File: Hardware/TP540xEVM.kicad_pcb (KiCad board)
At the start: 2 copper layers, 27.9 x 20.3 mm, 11 parts, among them U1 TPS5403

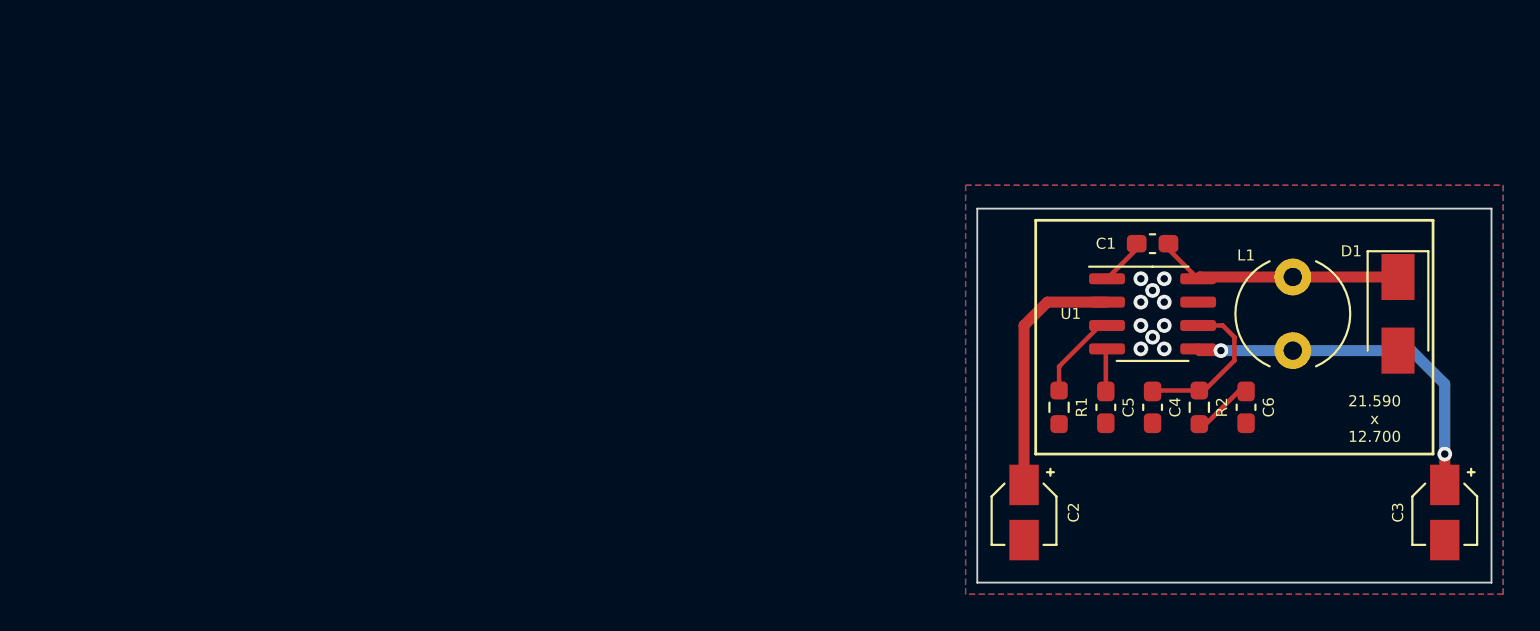
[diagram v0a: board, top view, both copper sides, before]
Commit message: ...
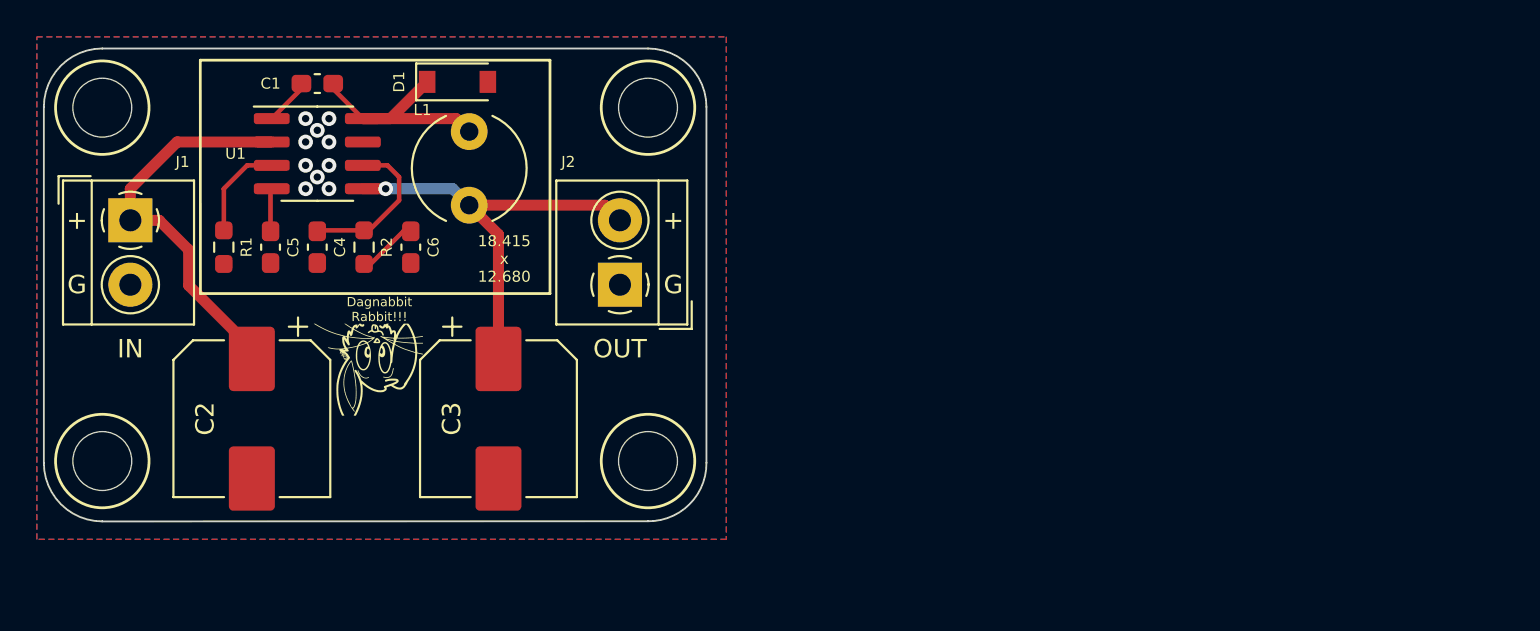
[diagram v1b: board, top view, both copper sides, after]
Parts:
- added J1: Input, TerminalBlock_4Ucon:TerminalBlock_4Ucon_1x02_P3.50mm_Horizontal, F.Cu at (86.7, 96.5)
- added J2: Output, TerminalBlock_4Ucon:TerminalBlock_4Ucon_1x02_P3.50mm_Horizontal, F.Cu at (113.3, 100.0)
- added REF**: Mount, Tinker:Mount, F.Cu at (114.8, 109.6)
- added REF**: Mount, Tinker:Mount, F.Cu at (85.2, 90.4)
- added REF**: Mount, Tinker:Mount, F.Cu at (85.2, 109.6)
- added REF**: DagNabbit, Tinker:DagNabbit, F.Cu at (99.9, 104.0)
- added REF**: Mount, Tinker:Mount, F.Cu at (114.8, 90.4)
- C2, C3: value 220uF -> 330uF; footprint Capacitor_SMD:CP_Elec_3x5.3 -> Capacitor_SMD:CP_Elec_8x10
- D1: value D_Schottky -> DSK24; footprint Diode_SMD:D_SMA -> Diode_SMD:D_SOD-123
- moved D1 52.6 mm to (104.5, 89.0), turned to 0 degrees
- moved C3 51.7 mm to (106.7, 107.3)
- moved C1 46.2 mm to (96.9, 89.1)
- moved C4 46.2 mm to (96.9, 98.0)
- moved R2 46.2 mm to (99.4, 98.0)
- moved U1 46.2 mm to (96.9, 92.9)
- moved C5 46.2 mm to (94.3, 98.0)
- moved C6 46.2 mm to (101.9, 98.0)
- moved R1 46.2 mm to (91.8, 98.0)
- moved L1 45.4 mm to (105.1, 91.7)
- moved C2 42.3 mm to (93.3, 107.3)
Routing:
- net Vin: track 13.7 -> 21.4 mm
- net Vout: track 19.7 -> 23.7 mm, vias 2 -> 1
- net Net-(R1-Pad1): track 4.83 -> 5.39 mm
- net Net-(C1-Pad2): track 13.5 -> 13.0 mm
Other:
- board size 27.9 x 20.3 mm -> 36 x 25.7 mm
- board text added: "+"
- board text added: "18.415 x 12.680"
- board text added: "G"
- board text added: "IN"
- board text added: "OUT"
- board text removed: "21.590 x 12.700"
